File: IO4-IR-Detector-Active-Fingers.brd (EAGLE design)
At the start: 103 x 107.4 mm, 32 parts, among them J1 0.100, J10 0.100, J11 0.100, J12 0.100, J13 0.100, J14 0.100, J15 0.100, J16 0.100, J2 0.100, J3 0.100, J4 0.100, J5 0.100, J6 0.100, J7 0.100, J8 0.100, J9 0.100, U1 QRE1113, U10 QRE1113, U11 QRE1113, U12 QRE1113, U13 QRE1113, U14 QRE1113, U15 QRE1113, U16 QRE1113, U2 QRE1113, U3 QRE1113, U4 QRE1113, U5 QRE1113, U6 QRE1113, U7 QRE1113, U8 QRE1113, U9 QRE1113

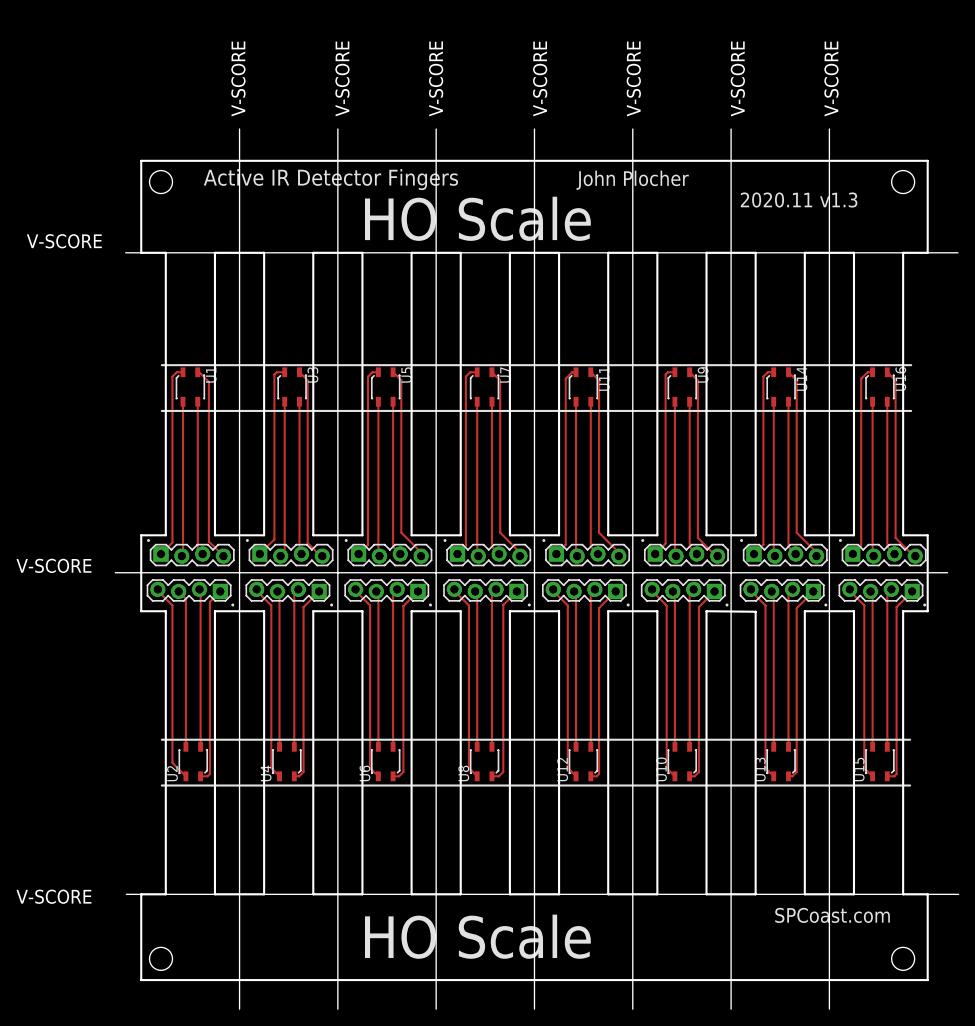
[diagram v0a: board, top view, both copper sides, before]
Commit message: N-Scale
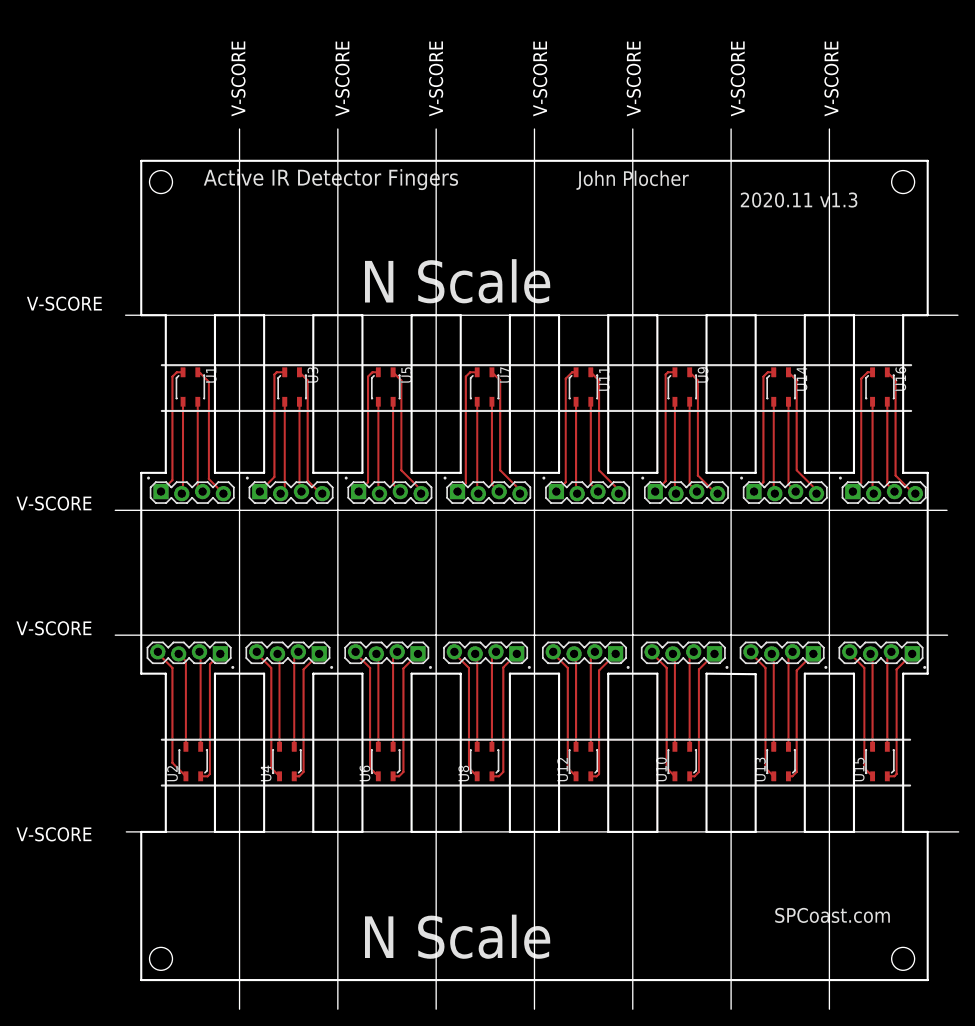
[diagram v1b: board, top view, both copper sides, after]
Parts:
- moved J1 7.62 mm to (2.41, 59.5)
- moved J11 7.62 mm to (50.7, 59.5)
- moved J14 7.62 mm to (74.8, 59.5)
- moved J16 7.62 mm to (86.9, 59.5)
- moved J3 7.62 mm to (14.5, 59.5)
- moved J5 7.62 mm to (26.5, 59.5)
- moved J7 7.62 mm to (38.6, 59.5)
- moved J9 7.62 mm to (62.7, 59.5)
- moved J10 7.62 mm to (70.0, 39.9)
- moved J12 7.62 mm to (57.9, 39.9)
- moved J13 7.62 mm to (82.0, 39.9)
- moved J15 7.62 mm to (94.1, 39.9)
- moved J2 7.62 mm to (9.65, 39.9)
- moved J4 7.62 mm to (21.7, 39.9)
- moved J6 7.62 mm to (33.8, 39.9)
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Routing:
- net N$59: track 19.4 -> 11.8 mm
- net N$58: track 24.0 -> 16.4 mm
- net N$54: track 19.4 -> 11.8 mm
- net N$53: track 24.0 -> 16.4 mm
- net N$52: track 19.4 -> 11.8 mm
- net N$5: track 19.4 -> 11.8 mm
- net N$46: track 19.4 -> 11.8 mm
- net N$45: track 24.0 -> 16.4 mm
- net N$4: track 24.0 -> 16.4 mm
- net N$36: track 19.4 -> 11.8 mm
- net N$35: track 24.0 -> 16.4 mm
- net N$30: track 19.4 -> 11.8 mm
- net N$29: track 24.0 -> 16.4 mm
- net N$19: track 24.2 -> 16.6 mm
- net N$20: track 19.3 -> 11.7 mm
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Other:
- outline, holes or cut-outs redrawn
- board text added: "N Scale"
- board text removed: "HO Scale"
